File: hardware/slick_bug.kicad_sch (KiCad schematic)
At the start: 8 parts, among them J1 Conn_01x04_Socket, J2 Conn_01x04_Socket, U1 XIAO-RP2040-SMD, U4 MAX40203AUK+T

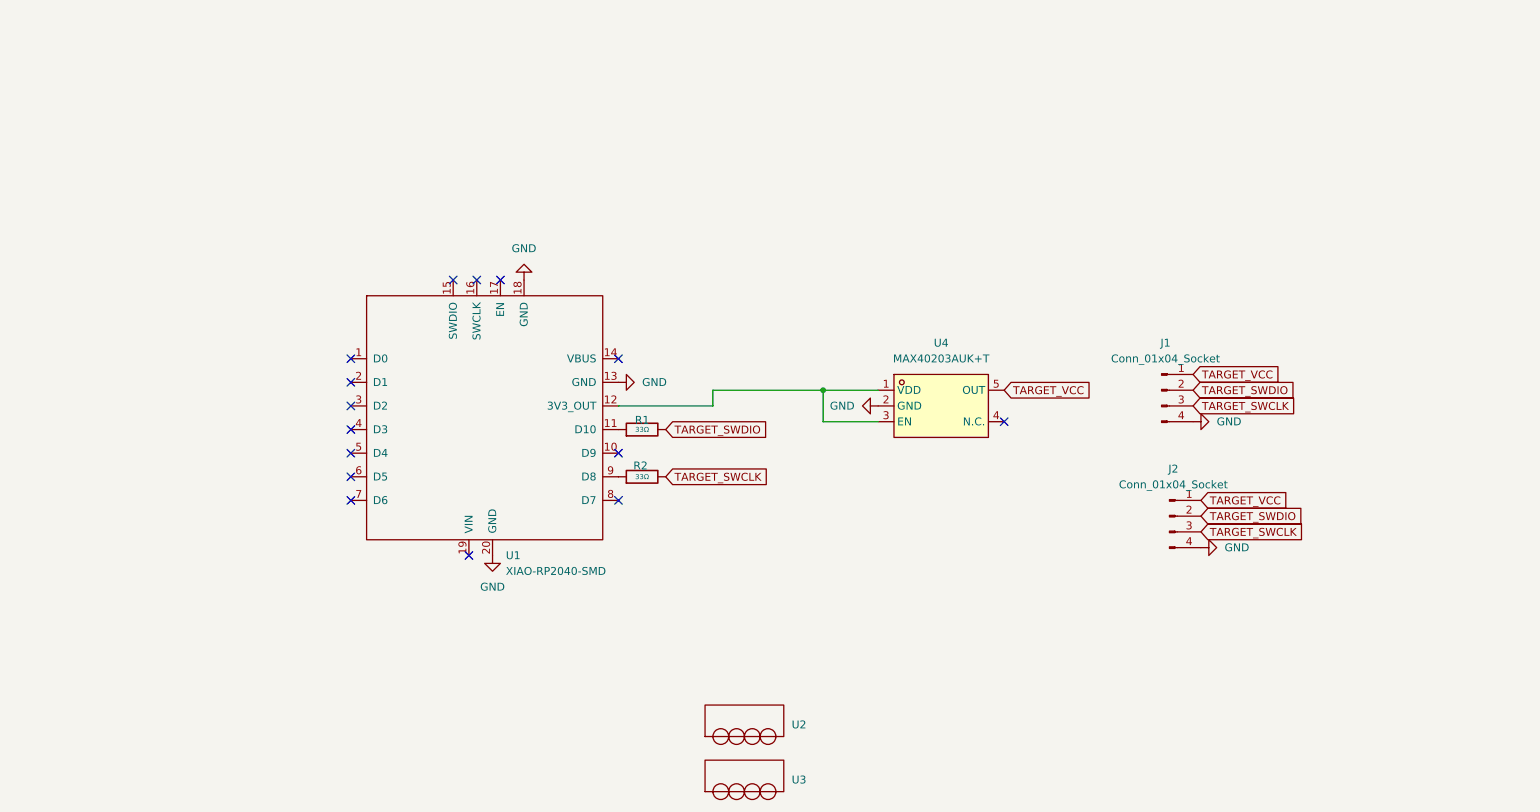
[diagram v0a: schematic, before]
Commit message: tweaks
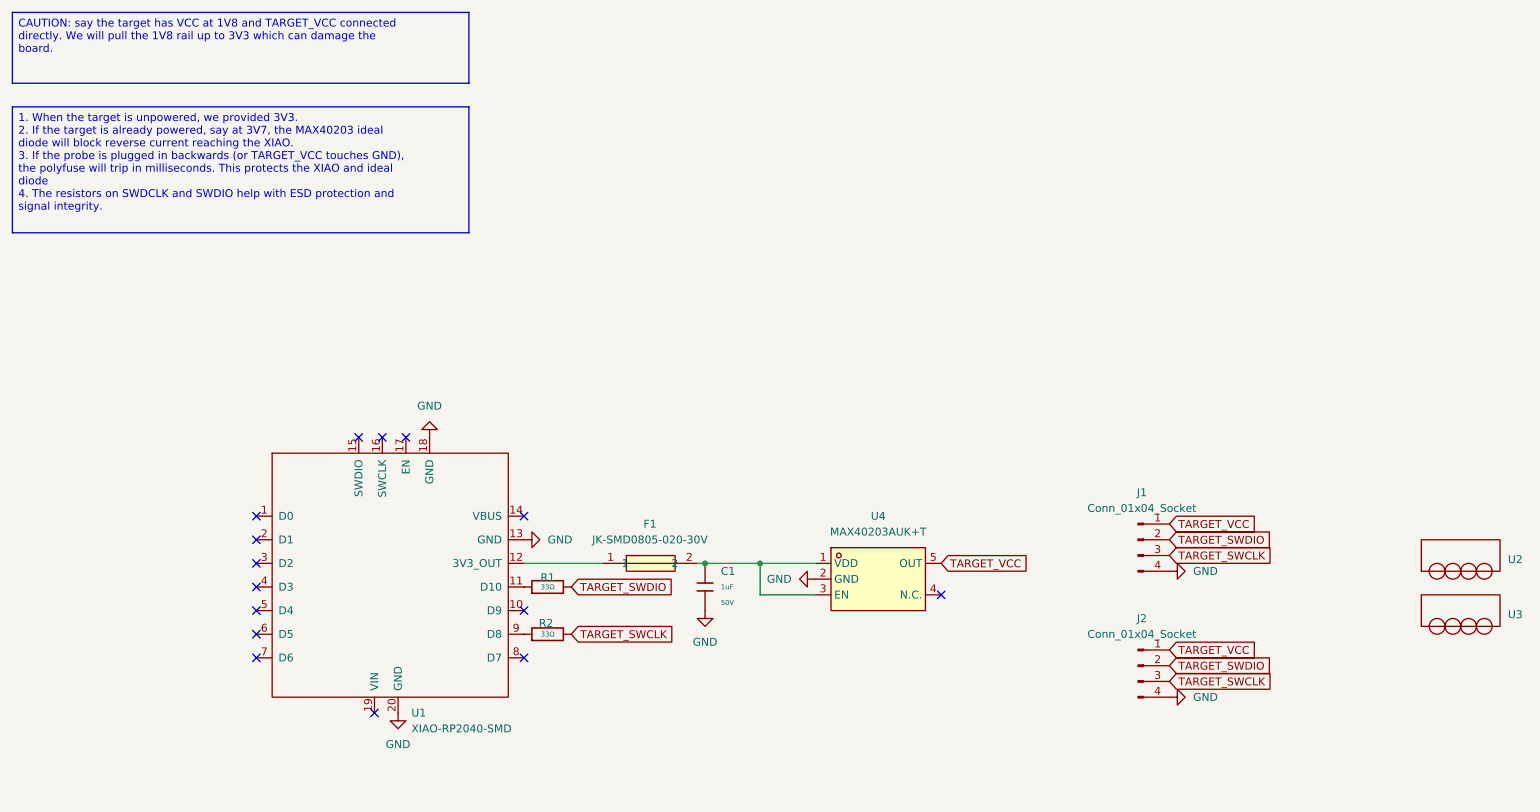
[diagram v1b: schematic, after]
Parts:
- added C1: 1uF, PCM_JLCPCB:C_0603, symbol PCM_JLCPCB-Capacitors:0603,1uF
- added F1: JK-SMD0805-020-30V, easyeda:F0805, symbol easyeda:JK-SMD0805-020-30V
- J2: footprint Connector_PinHeader_2.54mm:PinHeader_1x04_P2.54mm_Horizontal -> halfr:Harwin_M20-89004xx_1x04_P2.54mm_Horizontal_blank
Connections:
- net GND: now also C1.2
- net at U4.1 (VDD), U4.3 (EN): now also C1.1, F1.2; no longer U1.12 (3V3_OUT)
- new net: F1.1, U1.12 (3V3_OUT)
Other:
- moved on the sheet: J1, J2, R1, R2, U1, U2, U3, U4

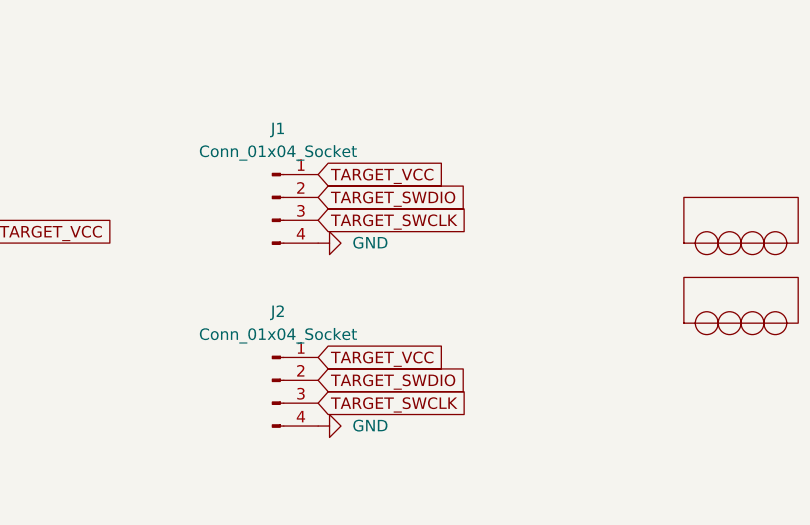
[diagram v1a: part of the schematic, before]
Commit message: pin order change
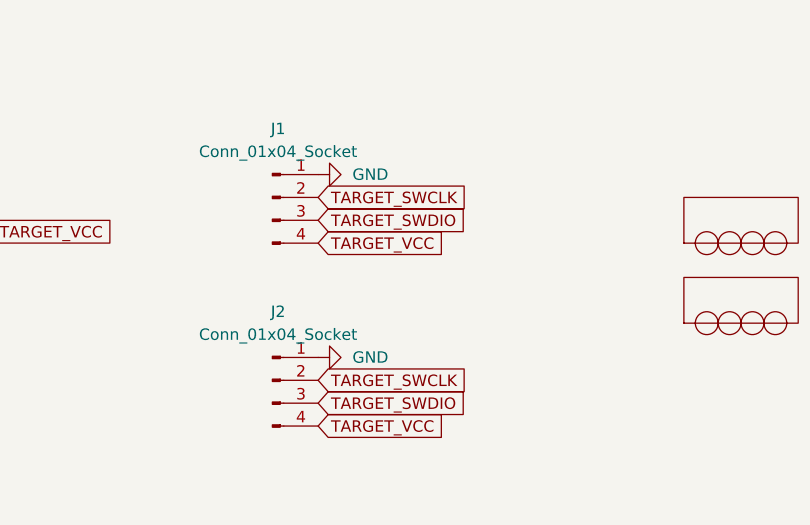
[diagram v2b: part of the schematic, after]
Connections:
- net GND: now also J1.1 (Pin_1), J2.1 (Pin_1); no longer J1.4 (Pin_4), J2.4 (Pin_4)
- net TARGET_SWCLK: now also J1.2 (Pin_2), J2.2 (Pin_2); no longer J1.3 (Pin_3), J2.3 (Pin_3)
- net TARGET_SWDIO: now also J1.3 (Pin_3), J2.3 (Pin_3); no longer J1.2 (Pin_2), J2.2 (Pin_2)
- net TARGET_VCC: now also J1.4 (Pin_4), J2.4 (Pin_4); no longer J1.1 (Pin_1), J2.1 (Pin_1)
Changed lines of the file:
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@@
 	(global_label "TARGET_SWCLK"
 		(shape input)
-		(at 200.66 123.19 0)
+		(at 200.66 120.65 0)
 		(fields_autoplaced yes)
 		(effects
@@
 		)
 		(property "Intersheetrefs" "${INTERSHEET_REFS}"
-			(at 217.5546 123.19 0)
+			(at 217.5546 120.65 0)
 			(hide yes)
 			(show_name no)
@@
 	(global_label "TARGET_SWCLK"
 		(shape input)
+		(at 200.66 100.33 0)
+		(fields_autoplaced yes)
+		(effects
+			(font
+				(size 1.27 1.27)
+			)
+			(justify left)
+		)
+		(property "Intersheetrefs" "${INTERSHEET_REFS}"
+			(at 217.5546 100.33 0)
+			(hide yes)
+			(show_name no)
+			(do_not_autoplace no)
+			(effects
+				(font
+					(size 1.27 1.27)
+				)
+				(justify left)
+			)
+		)
+	)
+	(global_label "TARGET_SWDIO"
+		(shape input)
 		(at 200.66 102.87 0)
 		(fields_autoplaced yes)
@@
 		)
 		(property "Intersheetrefs" "${INTERSHEET_REFS}"
-			(at 217.5546 102.87 0)
+			(at 217.1918 102.87 0)
 			(hide yes)
 			(show_name no)
@@
 		)
 	)
-	(global_label "TARGET_SWDIO"
+	(global_label "TARGET_VCC"
 		(shape input)
-		(at 200.66 100.33 0)
+		(at 200.66 105.41 0)
 		(fields_autoplaced yes)
 		(effects
@@
 		)
 		(property "Intersheetrefs" "${INTERSHEET_REFS}"
-			(at 217.1918 100.33 0)
+			(at 214.9542 105.41 0)
 			(hide yes)
 			(show_name no)
@@
 	(global_label "TARGET_VCC"
 		(shape input)
-		(at 200.66 97.79 0)
+		(at 200.66 125.73 0)
 		(fields_autoplaced yes)
 		(effects
@@
 		)
 		(property "Intersheetrefs" "${INTERSHEET_REFS}"
-			(at 214.9542 97.79 0)
+			(at 214.9542 125.73 0)
 			(hide yes)
 			(show_name no)
@@
 		)
 	)
-	(global_label "TARGET_VCC"
+	(global_label "TARGET_SWDIO"
 		(shape input)
-		(at 200.66 118.11 0)
+		(at 200.66 123.19 0)
 		(fields_autoplaced yes)
 		(effects
@@
 		)
 		(property "Intersheetrefs" "${INTERSHEET_REFS}"
-			(at 214.9542 118.11 0)
-			(hide yes)
-			(show_name no)
-			(do_not_autoplace no)
-			(effects
-				(font
-					(size 1.27 1.27)
-				)
-				(justify left)
-			)
-		)
-	)
-	(global_label "TARGET_SWDIO"
-		(shape input)
-		(at 200.66 120.65 0)
-		(fields_autoplaced yes)
-		(effects
-			(font
-				(size 1.27 1.27)
-			)
-			(justify left)
-		)
-		(property "Intersheetrefs" "${INTERSHEET_REFS}"
-			(at 217.1918 120.65 0)
+			(at 217.1918 123.19 0)
 			(hide yes)
 			(show_name no)
@@
 	(symbol
 		(lib_id "power:GND")
-		(at 200.66 105.41 90)
+		(at 200.66 97.79 90)
 		(mirror x)
 		(unit 1)
@@
 		(fields_autoplaced yes)
 		(property "Reference" "#PWR03"
-			(at 207.01 105.41 0)
+			(at 207.01 97.79 0)
 			(hide yes)
 			(show_name no)
@@
 		)
 		(property "Value" "GND"
-			(at 204.47 105.4099 90)
+			(at 204.47 97.7899 90)
 			(show_name no)
 			(do_not_autoplace no)
@@
 		)
 		(property "Footprint" ""
-			(at 200.66 105.41 0)
+			(at 200.66 97.79 0)
 			(hide yes)
 			(show_name no)
@@
 		)
 		(property "Datasheet" ""
-			(at 200.66 105.41 0)
+			(at 200.66 97.79 0)
 			(hide yes)
 			(show_name no)
@@
 		)
 		(property "Description" "Power symbol creates a global label with name \"GND\" , ground"
-			(at 200.66 105.41 0)
+			(at 200.66 97.79 0)
 			(hide yes)
 			(show_name no)
@@
 	(symbol
 		(lib_id "power:GND")
-		(at 200.66 125.73 90)
-		(mirror x)
+		(at 200.66 118.11 90)
 		(unit 1)
 		(body_style 1)
@@
 		(fields_autoplaced yes)
 		(property "Reference" "#PWR05"
-			(at 207.01 125.73 0)
+			(at 207.01 118.11 0)
 			(hide yes)
 			(show_name no)
@@
 		)
 		(property "Value" "GND"
-			(at 204.47 125.7299 90)
+			(at 204.47 118.1101 90)
 			(show_name no)
 			(do_not_autoplace no)
@@
 		)
 		(property "Footprint" ""
-			(at 200.66 125.73 0)
+			(at 200.66 118.11 0)
 			(hide yes)
 			(show_name no)
@@
 		)
 		(property "Datasheet" ""
-			(at 200.66 125.73 0)
+			(at 200.66 118.11 0)
 			(hide yes)
 			(show_name no)
@@
 		)
 		(property "Description" "Power symbol creates a global label with name \"GND\" , ground"
-			(at 200.66 125.73 0)
-			(hide yes)
-			(show_name no)
+			(at 200.66 118.11 0)
+			(hide yes)
+			(show_name no)

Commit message: slick bug
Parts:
- J1, J2, U1, U2, U3: now left out of the parts list
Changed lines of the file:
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@@
 		(body_style 1)
 		(exclude_from_sim no)
-		(in_bom yes)
+		(in_bom no)
 		(on_board yes)
 		(in_pos_files yes)
@@
 		(body_style 1)
 		(exclude_from_sim no)
-		(in_bom yes)
+		(in_bom no)
 		(on_board yes)
 		(in_pos_files yes)
@@
 		(body_style 1)
 		(exclude_from_sim no)
-		(in_bom yes)
+		(in_bom no)
 		(on_board yes)
 		(in_pos_files yes)
@@
 		(body_style 1)
 		(exclude_from_sim no)
-		(in_bom yes)
+		(in_bom no)
 		(on_board yes)
 		(in_pos_files yes)
@@
 		(body_style 1)
 		(exclude_from_sim no)
-		(in_bom yes)
+		(in_bom no)
 		(on_board yes)
 		(in_pos_files yes)

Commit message: move slick bug stuff to own folder
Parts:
- F1: footprint easyeda:F0805 -> slick_bug:F0805; symbol easyeda:JK-SMD0805-020-30V -> slick_bug:JK-SMD0805-020-30V
- J1: footprint halfr:R50_horizontal_4pin -> slick_bug:R50_horizontal_4pin
- J2: footprint halfr:Harwin_M20-89004xx_1x04_P2.54mm_Horizontal_blank -> slick_bug:Harwin_M20-89004xx_1x04_P2.54mm_Horizontal_blank
- U1: footprint Seeed_Studio_XIAO_Series:XIAO-RP2040-SMD -> slick_bug:XIAO-RP2040-SMD; symbol Seeed_Studio_XIAO_Series:XIAO-RP2040-SMD -> slick_bug:XIAO-RP2040-SMD
- U2, U3: footprint halfr:R50_pcb_comb -> slick_bug:R50_pcb_comb; symbol halfr:R50_pcb_comb -> slick_bug:R50_pcb_comb
- U4: footprint easyeda:SOT-23-5_L3.0-W1.6-P0.95-LS2.8-BR -> slick_bug:SOT-23-5_L3.0-W1.6-P0.95-LS2.8-BR; symbol easyeda:MAX40203AUK+T -> slick_bug:MAX40203AUK+T
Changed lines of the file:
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@@
 			)
 		)
-		(property "Footprint" "halfr:Harwin_M20-89004xx_1x04_P2.54mm_Horizontal_blank"
+		(property "Footprint" "slick_bug:Harwin_M20-89004xx_1x04_P2.54mm_Horizontal_blank"
 			(at 195.58 120.65 0)
 			(hide yes)
@@
 	)
 	(symbol
-		(lib_id "halfr:R50_pcb_comb")
+		(lib_id "slick_bug:R50_pcb_comb")
 		(at 247.65 107.95 0)
 		(unit 1)
@@
 			)
 		)
-		(property "Footprint" "halfr:R50_pcb_comb"
+		(property "Footprint" "slick_bug:R50_pcb_comb"
 			(at 247.65 107.95 0)
 			(hide yes)
@@
 	)
 	(symbol
-		(lib_id "halfr:R50_pcb_comb")
+		(lib_id "slick_bug:R50_pcb_comb")
 		(at 247.65 99.06 0)
 		(unit 1)
@@
 			)
 		)
-		(property "Footprint" "halfr:R50_pcb_comb"
+		(property "Footprint" "slick_bug:R50_pcb_comb"
 			(at 247.65 99.06 0)
 			(hide yes)
@@
 	)
 	(symbol
-		(lib_id "easyeda:JK-SMD0805-020-30V")
+		(lib_id "slick_bug:JK-SMD0805-020-30V")
 		(at 116.84 104.14 0)
 		(unit 1)
@@
 			)
 		)
-		(property "Footprint" "easyeda:F0805"
+		(property "Footprint" "slick_bug:F0805"
 			(at 116.84 111.76 0)
 			(hide yes)
@@
 	)
 	(symbol
-		(lib_id "easyeda:MAX40203AUK+T")
+		(lib_id "slick_bug:MAX40203AUK+T")
 		(at 153.67 106.68 0)
 		(unit 1)
@@
 			)
 		)
-		(property "Footprint" "easyeda:SOT-23-5_L3.0-W1.6-P0.95-LS2.8-BR"
+		(property "Footprint" "slick_bug:SOT-23-5_L3.0-W1.6-P0.95-LS2.8-BR"
 			(at 153.67 116.84 0)
 			(hide yes)
@@
 			)
 		)
-		(property "Footprint" "halfr:R50_horizontal_4pin"
+		(property "Footprint" "slick_bug:R50_horizontal_4pin"
 			(at 195.58 100.33 0)
 			(hide yes)
@@
 	)
 	(symbol
-		(lib_id "Seeed_Studio_XIAO_Series:XIAO-RP2040-SMD")
+		(lib_id "slick_bug:XIAO-RP2040-SMD")
 		(at 74.93 97.79 0)
 		(unit 1)
@@
 			)
 		)
-		(property "Footprint" "Seeed_Studio_XIAO_Series:XIAO-RP2040-SMD"
+		(property "Footprint" "slick_bug:XIAO-RP2040-SMD"
 			(at 79.248 127.762 0)
 			(hide yes)
